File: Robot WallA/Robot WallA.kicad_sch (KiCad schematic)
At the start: 4 parts

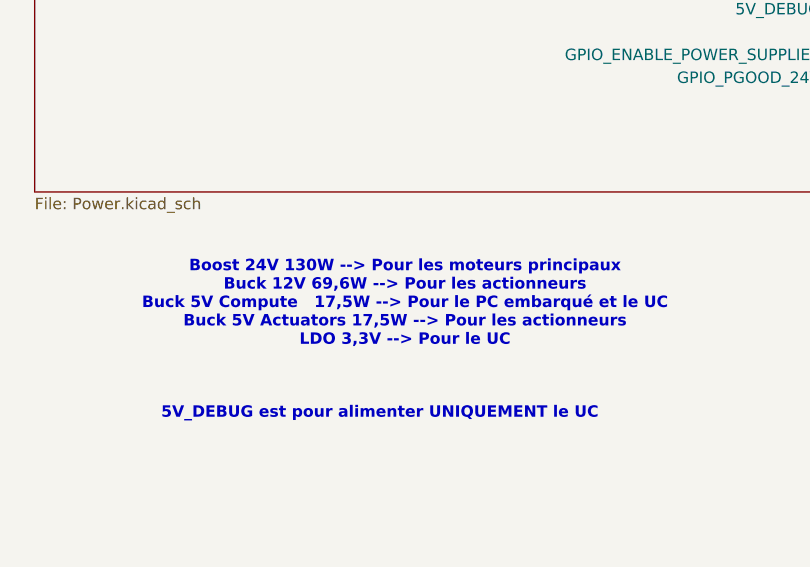
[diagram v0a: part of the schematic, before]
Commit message: Reworked 12V and 5V power supplies, continue routing
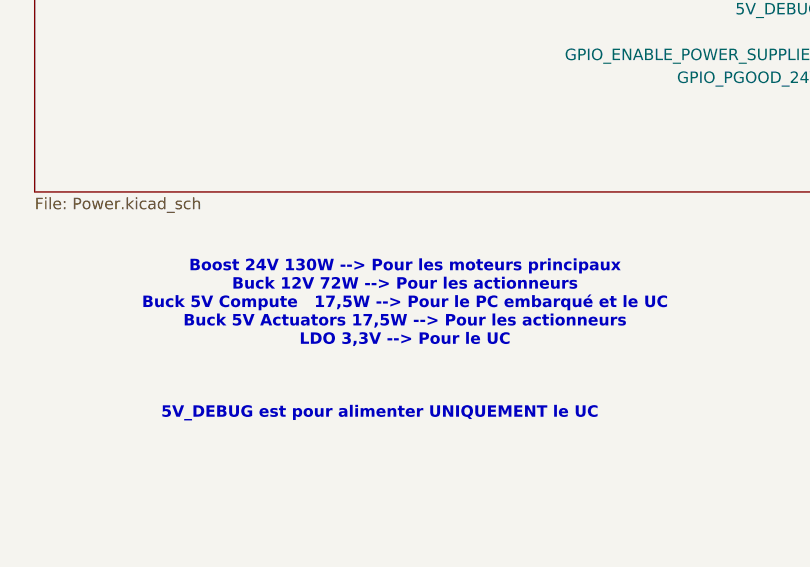
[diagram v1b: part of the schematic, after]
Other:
- note added: "Boost 24V 130W --> Pour les moteurs principaux Buck 12V 72W --> Pour les actionneurs Buck 5V Compute 17,5W --> Pour le PC embarqué et le UC Buck 5V Actuators 17,5W --> Pour les actionneurs LDO 3,3V --> Pour le UC"
- note removed: "Boost 24V 130W --> Pour les moteurs principaux Buck 12V 69,6W --> Pour les actionneurs Buck 5V Compute 17,5W --> Pour le PC embarqué et le UC Buck 5V Actuators 17,5W --> Pour les actionneurs LDO 3,3V --> Pour le UC"
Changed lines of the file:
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@@
 		)
 	)
-	(text "Boost 24V 130W --> Pour les moteurs principaux\nBuck 12V 69,6W --> Pour les actionneurs\nBuck 5V Compute   17,5W --> Pour le PC embarqué et le UC\nBuck 5V Actuators 17,5W --> Pour les actionneurs\nLDO 3,3V --> Pour le UC"
+	(text "Boost 24V 130W --> Pour les moteurs principaux\nBuck 12V 72W --> Pour les actionneurs\nBuck 5V Compute   17,5W --> Pour le PC embarqué et le UC\nBuck 5V Actuators 17,5W --> Pour les actionneurs\nLDO 3,3V --> Pour le UC"
 		(exclude_from_sim no)
 		(at 61.468 73.406 0)
